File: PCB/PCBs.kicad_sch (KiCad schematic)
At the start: 22 parts, among them CN1 W2A41C681KAT2A, CN2 W2A41C681KAT2A, CN4 W2A41C681KAT2A, CN5 W2A41C681KAT2A, CN6 W2A41C681KAT2A, U1 ADS1299IPAGR, U3 TPD4E1B06DCKR, U4 TPD4E1B06DCKR, U6 TPD4E1B06DCKR

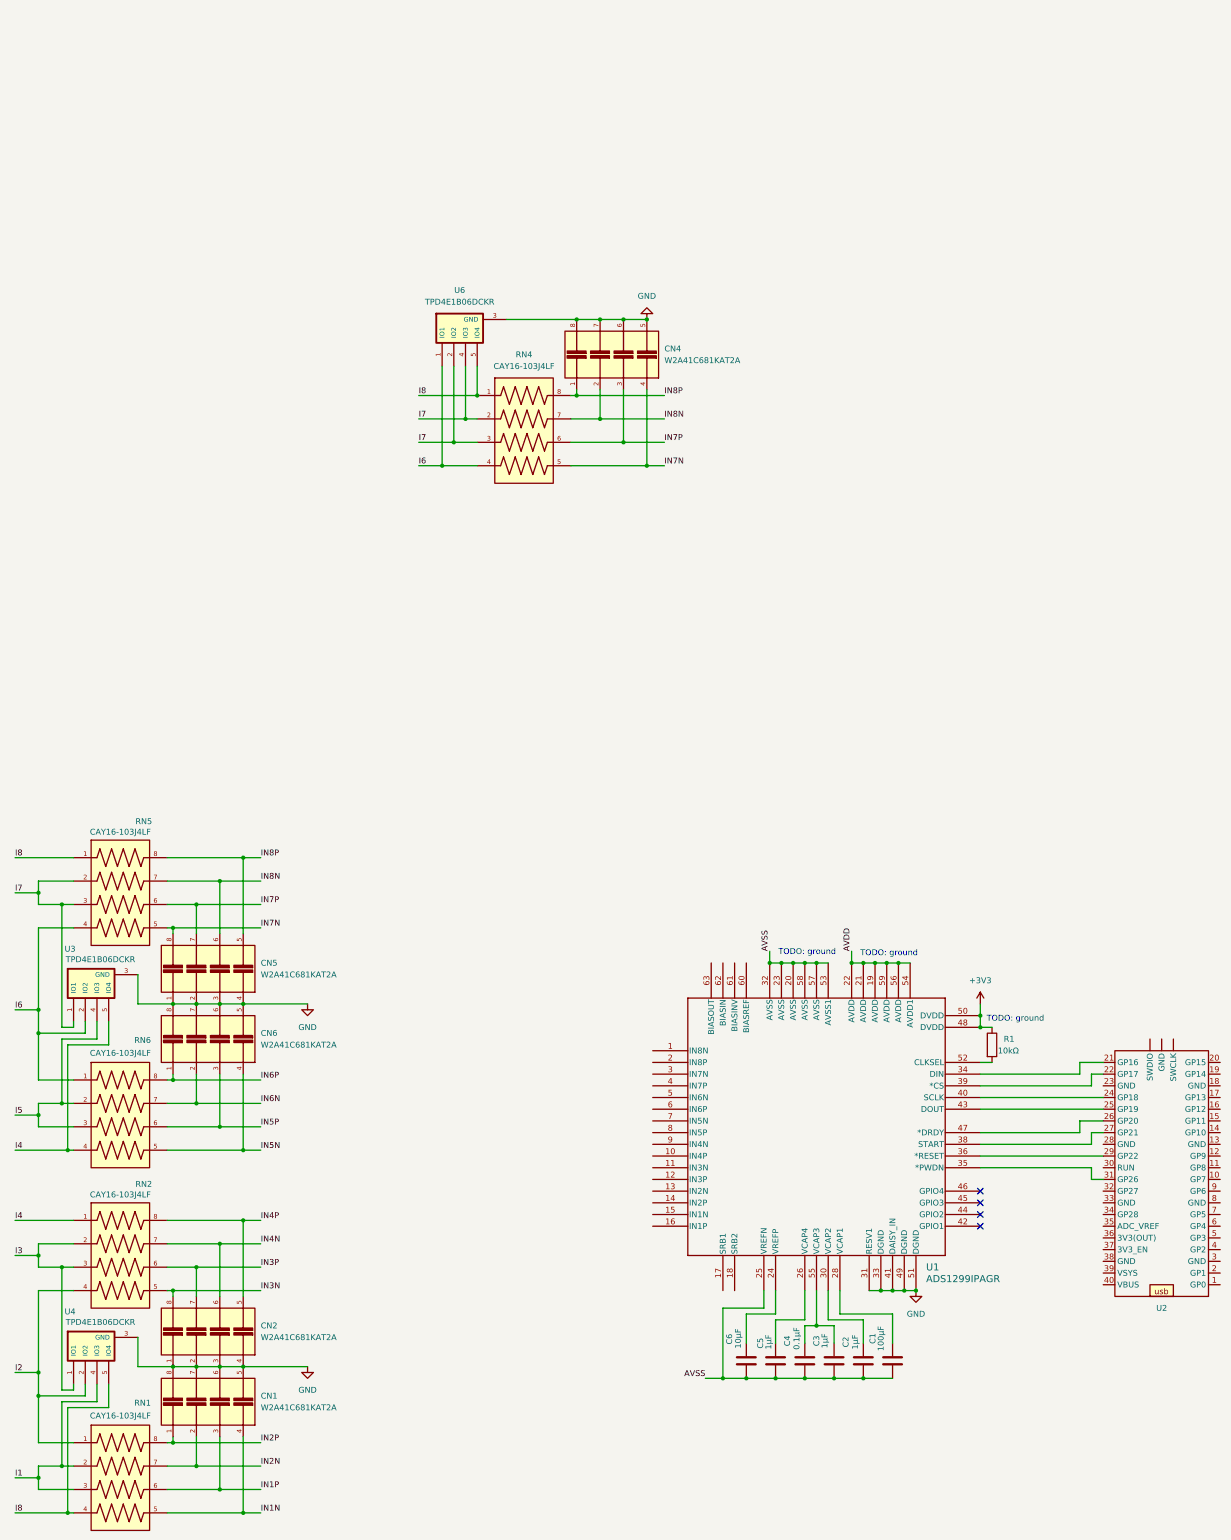
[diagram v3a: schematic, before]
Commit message: bias input draft
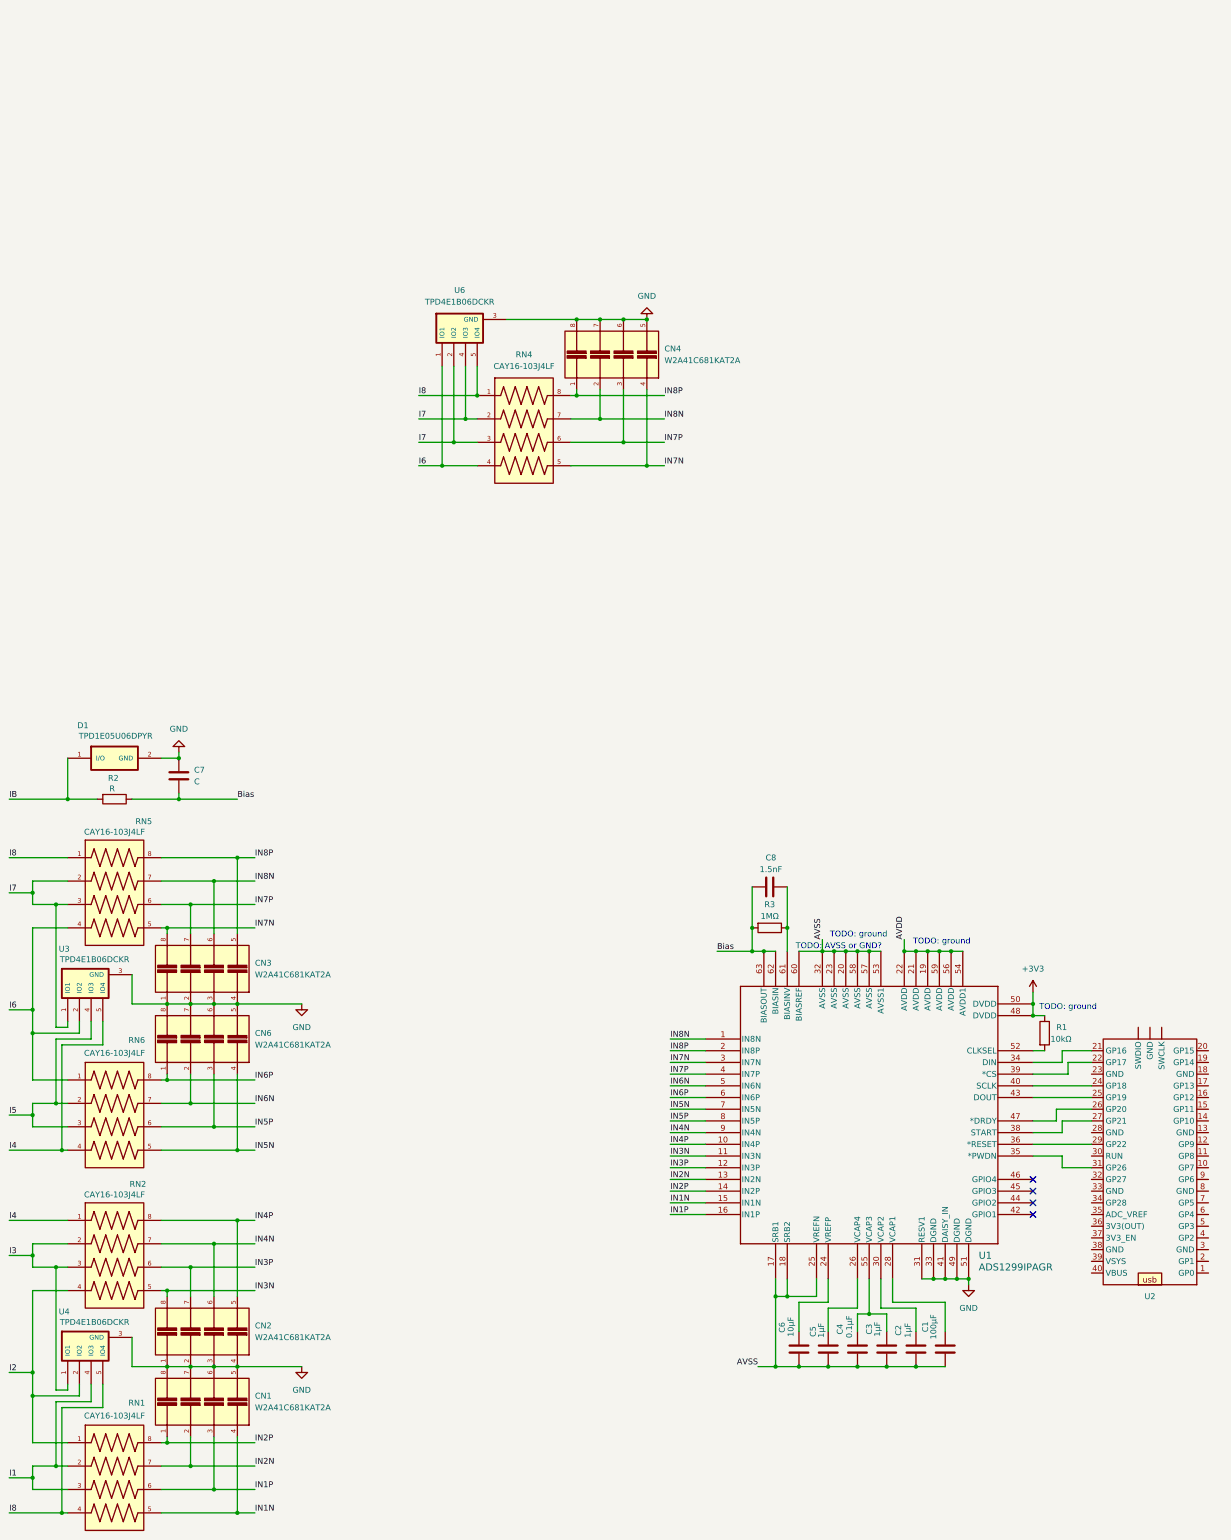
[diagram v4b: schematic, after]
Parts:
- removed CN5: W2A41C681KAT2A, W2A41C681KAT2A:CAPCAXE50P210X130X94-8N, symbol custom_lib:W2A41C681KAT2A
- added C7: C, symbol Device:C
- added C8: 1.5nF, symbol Device:C
- added CN3: W2A41C681KAT2A, W2A41C681KAT2A:CAPCAXE50P210X130X94-8N, symbol custom_lib:W2A41C681KAT2A
- added D1: TPD1E05U06DPYR, TPD1E05U06DPYR:DIO_TPD1E05U06DPYR, symbol custom_lib:TPD1E05U06DPYR
- added R2: R, symbol Device:R
- added R3: 1MΩ, symbol Device:R
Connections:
- net AVSS: now also U1.17 (SRB1), U1.18 (SRB2), U1.60 (BIASREF)
- net GND: now also C7.1, CN3.1, CN3.2, CN3.3, CN3.4, D1.2 (GND)
- net IN1N: now also U1.15 (IN1N)
- net IN1P: now also U1.16 (IN1P)
- net IN2N: now also U1.13 (IN2N)
- net IN2P: now also U1.14 (IN2P)
- net IN3N: now also U1.11 (IN3N)
- net IN3P: now also U1.12 (IN3P)
- net IN4N: now also U1.9 (IN4N)
- net IN4P: now also U1.10 (IN4P)
- net IN5N: now also U1.7 (IN5N)
- net IN5P: now also U1.8 (IN5P)
- net IN6N: now also U1.5 (IN6N)
- net IN6P: now also U1.6 (IN6P)
- net IN7N: now also U1.3 (IN7N), CN3.8
- net IN7P: now also U1.4 (IN7P), CN3.7
- net IN8N: now also U1.1 (IN8N), CN3.6
- net IN8P: now also U1.2 (IN8P), CN3.5
- net at U1.61 (BIASINV): now also C8.1, R3.1
- net Bias: now reaches U1.62 (BIASIN)
- net Bias: now also U1.63 (BIASOUT), C7.2, C8.2, R2.1, R3.2
- new net IB: D1.1 (I/O), R2.2
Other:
- note added: "TODO: AVSS or GND?"
- moved on the sheet: C1, C2, C3, C4, C5, C6, CN1, CN2, CN6, R1, RN1, RN2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
